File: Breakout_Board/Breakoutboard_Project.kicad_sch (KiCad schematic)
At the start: 17 parts, among them J1 Conn_01x17, J2 Conn_01x17, J3 Conn_01x17, J4 Conn_01x17, U2 STM32F411

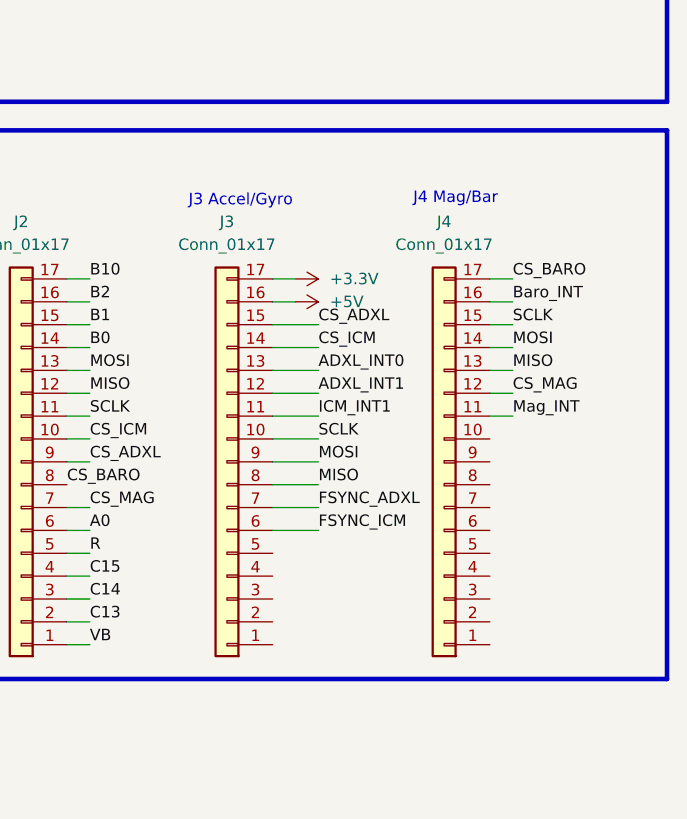
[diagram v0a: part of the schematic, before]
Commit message: some layout
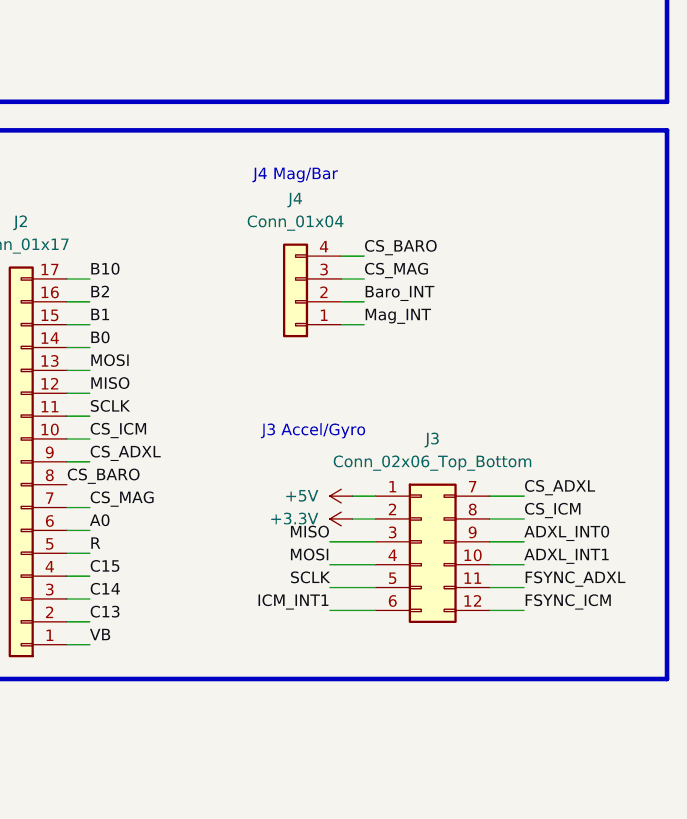
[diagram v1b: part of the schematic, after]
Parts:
- removed J3, J4: Conn_01x17, Package_QFP:LQFP-176_24x24mm_P0.5mm, symbol Connector_Generic:Conn_01x17
- added J3: Conn_02x06_Top_Bottom, Connector_PinHeader_1.27mm:PinHeader_2x06_P1.27mm_Vertical, symbol Connector_Generic:Conn_02x06_Top_Bottom
- added J4: Conn_01x04, Connector_PinSocket_2.54mm:PinSocket_1x04_P2.54mm_Vertical, symbol Connector_Generic:Conn_01x04
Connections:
- net +3.3V: now also J3.2 (Pin_2)
- net +5V: now also J3.1 (Pin_1)
- net ADXL_INT0: now also J3.9 (Pin_9)
- net ADXL_INT1: now also J3.10 (Pin_10)
- net Baro_INT: now also J4.2 (Pin_2)
- net CS_ADXL: now also J3.7 (Pin_7)
- net CS_BARO: now also J4.4 (Pin_4)
- net CS_ICM: now also J3.8 (Pin_8)
- net CS_MAG: now also J4.3 (Pin_3)
- net FSYNC_ADXL: now also J3.11 (Pin_11)
- net FSYNC_ICM: now also J3.12 (Pin_12)
- net ICM_INT1: now also J3.6 (Pin_6)
- net MISO: now also J3.3 (Pin_3)
- net MOSI: now also J3.4 (Pin_4)
- net Mag_INT: now also J4.1 (Pin_1)
- net SCLK: now also J3.5 (Pin_5)
